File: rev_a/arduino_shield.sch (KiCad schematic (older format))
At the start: 9 parts

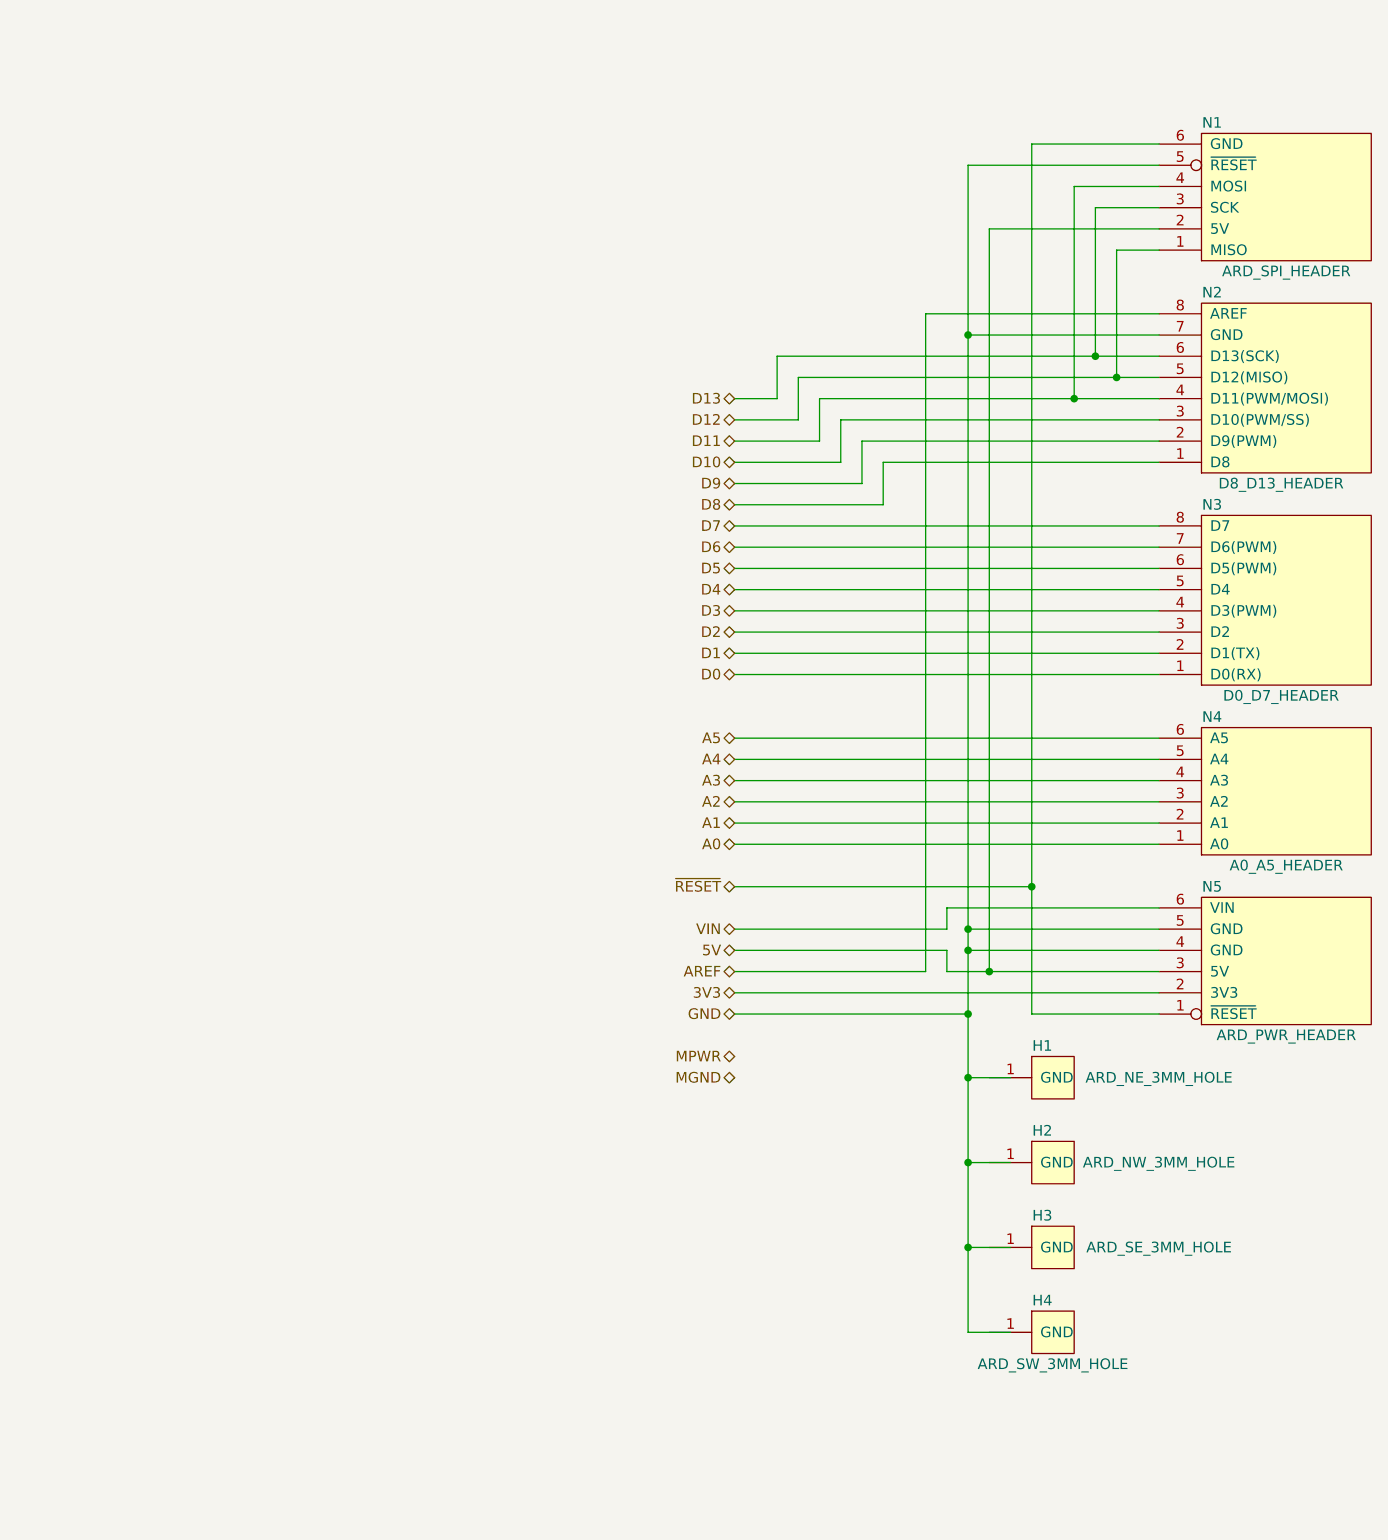
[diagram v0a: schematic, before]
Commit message: Rev. A of the Busino board layout is in pretty good shape.
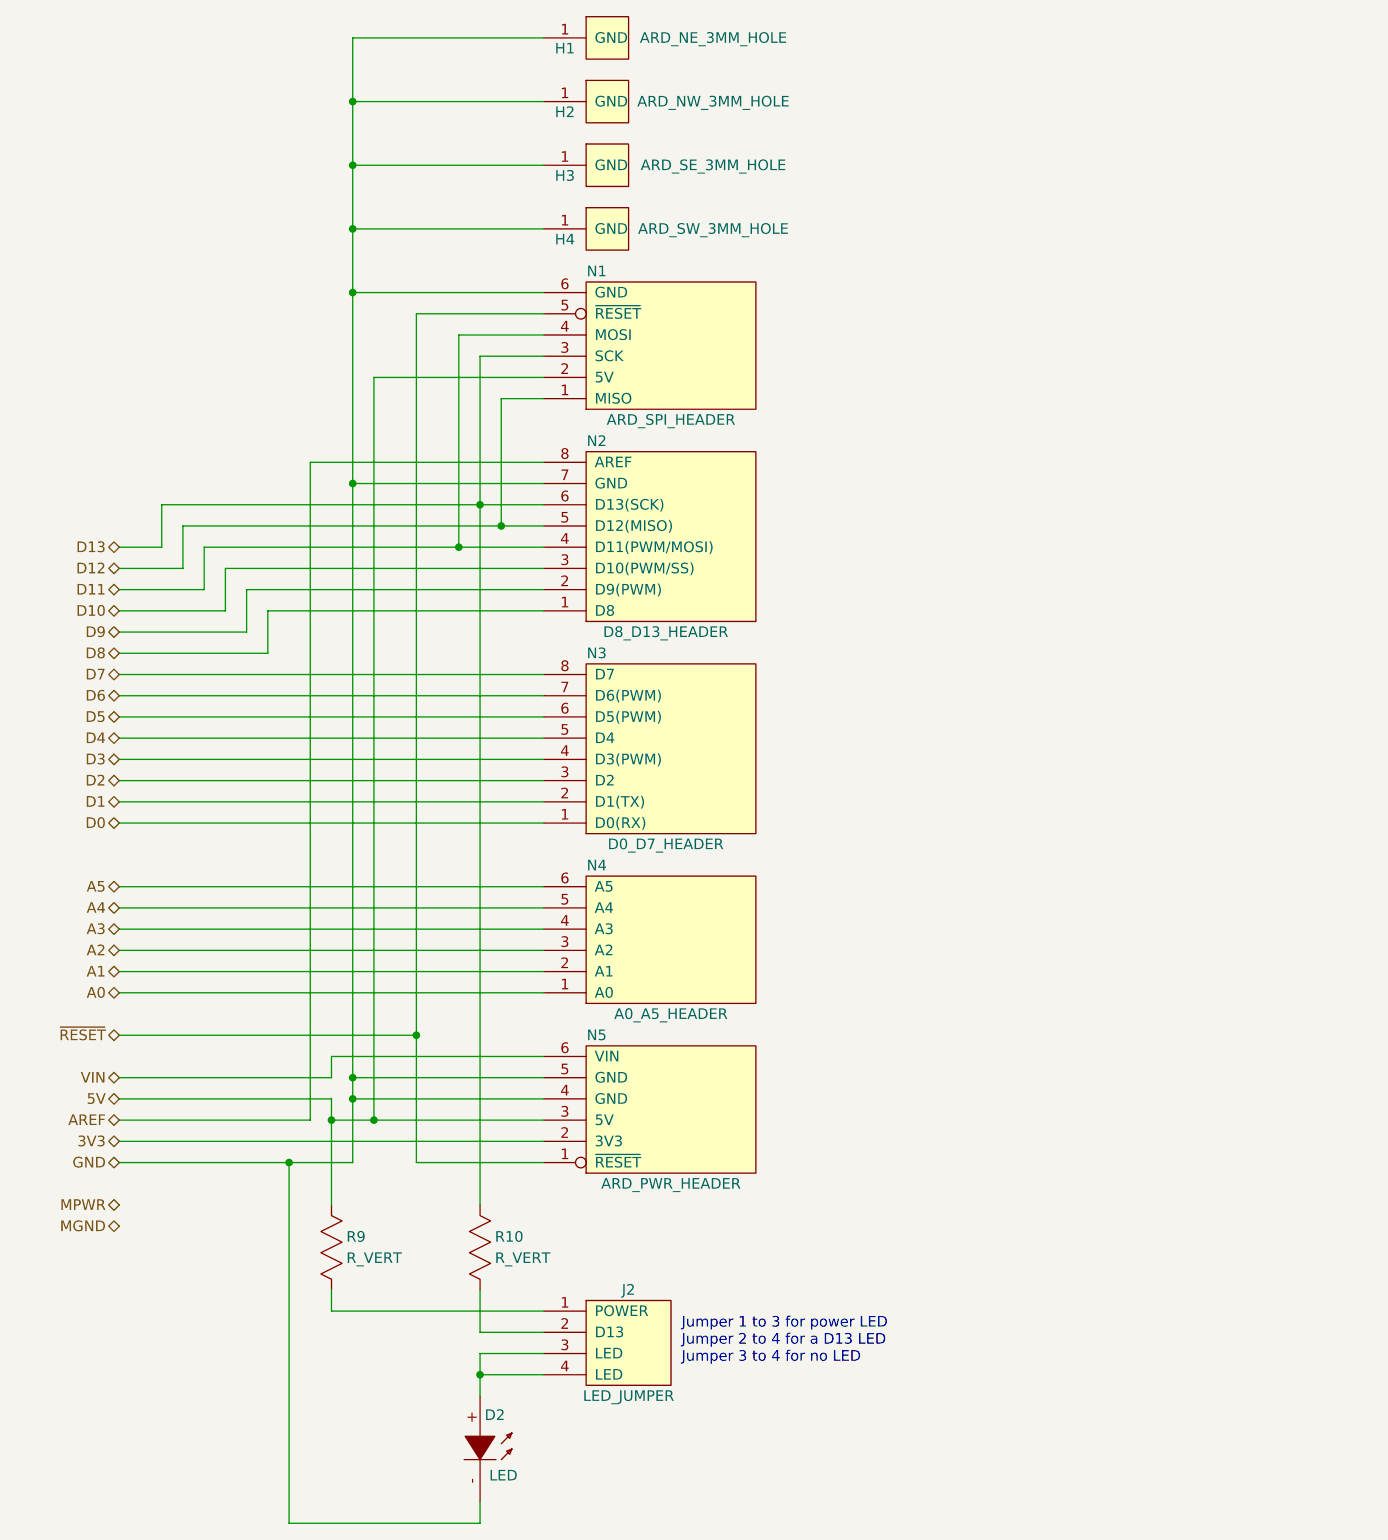
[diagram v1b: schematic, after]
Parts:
- added D2: LED, symbol LED
- added J2: LED_JUMPER, symbol LED_JUMPER
- added R10, R9: R_VERT, symbol R_VERT
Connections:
- wire segments 64 -> 74
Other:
- note added: "Jumper 1 to 3 for power LED\nJumper 2 to 4 for a D13 LED\nJumper 3 to 4 for no LED"
- moved on the sheet: H1, H2, H3, H4, N1, N2, N3, N4, N5
